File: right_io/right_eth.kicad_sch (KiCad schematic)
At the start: 29 parts, among them J500 JXD1-1022NL recessed 1GbE RJ45, U500 RTL8111H-CG-RH PCIe Gigabit E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, U501 D3V3XA4B10LP-7 four-channel 0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, U502 D3V3XA4B10LP-7 four-channel 0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, Y500 ECS-250-8-33-AGN-TR 25MHz 8pF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

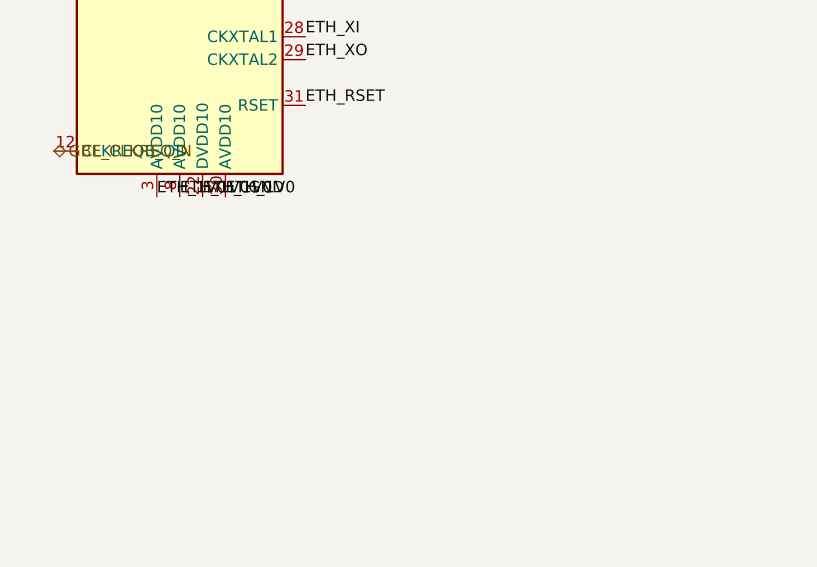
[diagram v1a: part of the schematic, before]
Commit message: fix the center layout and more board issues
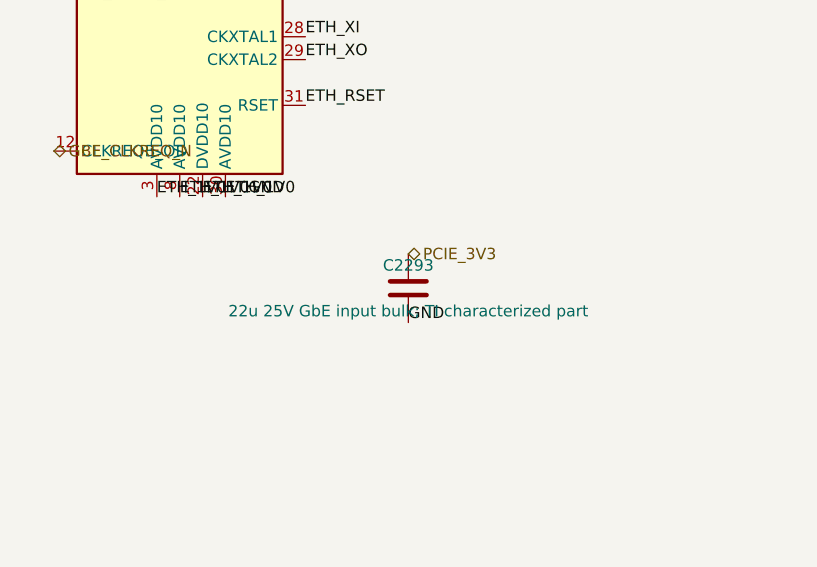
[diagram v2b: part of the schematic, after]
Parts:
- added C2293: 22u 25V GbE input bulk; TI characterized part, Capacitor_SMD:C_1210_3225Metric, symbol Device:C
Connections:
- net GND: now also C2293.2
- net PCIE_3V3: now also C2293.1
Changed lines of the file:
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@@
   (pin "33")
   (instances
-    (project "right_io"
+    (project "ducktop2"
       (path "/96046257-06f2-5617-bab9-b080ec1492e1"
         (reference "U500")
@@
   (pin "2")
   (instances
-    (project "right_io"
+    (project "ducktop2"
       (path "/96046257-06f2-5617-bab9-b080ec1492e1"
         (reference "C500")
@@
   (pin "2")
   (instances
-    (project "right_io"
+    (project "ducktop2"
       (path "/96046257-06f2-5617-bab9-b080ec1492e1"
         (reference "C501")
@@
   (pin "2")
   (instances
-    (project "right_io"
+    (project "ducktop2"
       (path "/96046257-06f2-5617-bab9-b080ec1492e1"
         (reference "C502")
@@
   (pin "2")
   (instances
-    (project "right_io"
+    (project "ducktop2"
       (path "/96046257-06f2-5617-bab9-b080ec1492e1"
         (reference "C503")
@@
   (pin "2")
   (instances
-    (project "right_io"
+    (project "ducktop2"
       (path "/96046257-06f2-5617-bab9-b080ec1492e1"
         (reference "C504")
@@
   (pin "2")
   (instances
-    (project "right_io"
+    (project "ducktop2"
       (path "/96046257-06f2-5617-bab9-b080ec1492e1"
         (reference "C505")
@@
   (pin "2")
   (instances
-    (project "right_io"
+    (project "ducktop2"
       (path "/96046257-06f2-5617-bab9-b080ec1492e1"
         (reference "C506")
@@
   (pin "2")
   (instances
-    (project "right_io"
+    (project "ducktop2"
       (path "/96046257-06f2-5617-bab9-b080ec1492e1"
         (reference "C507")
@@
   (pin "2")
   (instances
-    (project "right_io"
+    (project "ducktop2"
       (path "/96046257-06f2-5617-bab9-b080ec1492e1"
         (reference "C508")
@@
   (pin "2")
   (instances
-    (project "right_io"
+    (project "ducktop2"
       (path "/96046257-06f2-5617-bab9-b080ec1492e1"
         (reference "C509")
@@
   (pin "2")
   (instances
-    (project "right_io"
+    (project "ducktop2"
       (path "/96046257-06f2-5617-bab9-b080ec1492e1"
         (reference "C510")
@@
   (pin "2")
   (instances
-    (project "right_io"
+    (project "ducktop2"
       (path "/96046257-06f2-5617-bab9-b080ec1492e1"
         (reference "C511")
@@
   (pin "2")
   (instances
-    (project "right_io"
+    (project "ducktop2"
       (path "/96046257-06f2-5617-bab9-b080ec1492e1"
         (reference "C512")
@@
   (pin "2")
   (instances
-    (project "right_io"
+    (project "ducktop2"
       (path "/96046257-06f2-5617-bab9-b080ec1492e1"
         (reference "R501")
@@
   (pin "2")
   (instances
-    (project "right_io"
+    (project "ducktop2"
       (path "/96046257-06f2-5617-bab9-b080ec1492e1"
         (reference "R502")
@@
   (pin "2")
   (instances
-    (project "right_io"
+    (project "ducktop2"
       (path "/96046257-06f2-5617-bab9-b080ec1492e1"
         (reference "R503")
@@
   (pin "4")
   (instances
-    (project "right_io"
+    (project "ducktop2"
       (path "/96046257-06f2-5617-bab9-b080ec1492e1"
         (reference "Y500")
@@
   (pin "2")
   (instances
-    (project "right_io"
+    (project "ducktop2"
       (path "/96046257-06f2-5617-bab9-b080ec1492e1"
         (reference "R500")
@@
   (pin "2")
   (instances
-    (project "right_io"
+    (project "ducktop2"
       (path "/96046257-06f2-5617-bab9-b080ec1492e1"
         (reference "C515")
@@
   (pin "2")
   (instances
-    (project "right_io"
+    (project "ducktop2"
       (path "/96046257-06f2-5617-bab9-b080ec1492e1"
         (reference "C516")
@@
   (pin "10")
   (instances
-    (project "right_io"
+    (project "ducktop2"
       (path "/96046257-06f2-5617-bab9-b080ec1492e1"
         (reference "U501")
@@
   (pin "10")
   (instances
-    (project "right_io"
+    (project "ducktop2"
       (path "/96046257-06f2-5617-bab9-b080ec1492e1"
         (reference "U502")
@@
   (pin "SH")
   (instances
-    (project "right_io"
+    (project "ducktop2"
       (path "/96046257-06f2-5617-bab9-b080ec1492e1"
         (reference "J500")
@@
   (pin "2")
   (instances
-    (project "right_io"
+    (project "ducktop2"
       (path "/96046257-06f2-5617-bab9-b080ec1492e1"
         (reference "C513")
@@
   (pin "2")
   (instances
-    (project "right_io"
+    (project "ducktop2"
       (path "/96046257-06f2-5617-bab9-b080ec1492e1"
         (reference "R504")
@@
   (pin "2")
   (instances
-    (project "right_io"
+    (project "ducktop2"
       (path "/96046257-06f2-5617-bab9-b080ec1492e1"
         (reference "R505")
@@
   (pin "2")
   (instances
-    (project "right_io"
+    (project "ducktop2"
       (path "/96046257-06f2-5617-bab9-b080ec1492e1"
         (reference "C514")
@@
   (pin "2")
   (instances
-    (project "right_io"
+    (project "ducktop2"
       (path "/96046257-06f2-5617-bab9-b080ec1492e1"
         (reference "R506")
@@
 (text "ASSEMBLY HOLD: ask the assembler to confirm through-hole mid-mount RJ45 support and whether J500 is manual/post-reflow insertion." (at 20.32 381 0) (effects (font (size 1.27 1.27))))
 (text "LED HOLD: RTL8111H pin 26 is the default 1000M indication, not a generic link LED. Verify both jack LEDs at 10/100/1000 on hardware." (at 20.32 388.62 0) (effects (font (size 1.27 1.27))))
+(symbol
+  (lib_id "Device:C")
+  (at 304.8 199.39 0)
+  (unit 1)
+  (exclude_from_sim no)
+  (in_bom yes)
+  (on_board yes)
+  (dnp no)
+  (property "Reference" "C2293" (at 304.8 196.85 0) (effects (font (size 1.27 1.27))))
+  (property "Value" "22u 25V GbE input bulk; TI characterized part" (at 304.8 201.93 0) (effects (font (size 1.27 1.27))))
+  (property "Footprint" "Capacitor_SMD:C_1210_3225Metric" (at 304.8 199.39 0) (effects (font (size 1.27 1.27)) (hide yes)))
+  (property "Datasheet" "" (at 304.8 199.39 0) (effects (font (size 1.27 1.27)) (hide yes)))
+  (property "Manufacturer" "Murata" (at 304.8 199.39 0) (effects (font (size 1.27 1.27)) (hide yes)))
+  (property "MPN" "GRM32ER71E226KE15L" (at 304.8 199.39 0) (effects (font (size 1.27 1.27)) (hide yes)))
+  (property "Layout" "near_U500_3V3_pins;continuous_ground_plane;GbE_return_paired_with_loom_pin5" (at 304.8 199.39 0) (effects (font (size 1.27 1.27)) (hide yes)))
+  (pin "1")
+  (pin "2")
+  (instances
+    (project "ducktop2"
+      (path "/96046257-06f2-5617-bab9-b080ec1492e1"
+        (reference "C2293")
+        (unit 1)
+      )
+    )
+  )
+)
+(hierarchical_label "PCIE_3V3"
+  (shape bidirectional)
+  (at 304.8 195.58 0)
+  (effects (font (size 1.27 1.27)) (justify left bottom))
+)
+(label "GND"
+  (at 304.8 203.2 0)
+  (effects (font (size 1.27 1.27)) (justify left bottom))
+)
 (sheet_instances
   (path "/96046257-06f2-5617-bab9-b080ec1492e1"
